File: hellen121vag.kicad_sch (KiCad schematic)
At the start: 35 parts, among them J21 Conn_01x05_Male, J22 USB_B_Mini, M1 Module-power_12and5V-0.3, M2 Module-knock-0.2, M3 Module-vr-discrete-0.5, M4 Module-vr-max9924-0.1, M5 Module-wbo-0.5, M6 Module:mega-mcu100/0.3, M7 Module-can-0.1, M8 Module-motor-driver-0.1, P1 368255-2, Q7 AO3400A, U10 BTS6143D

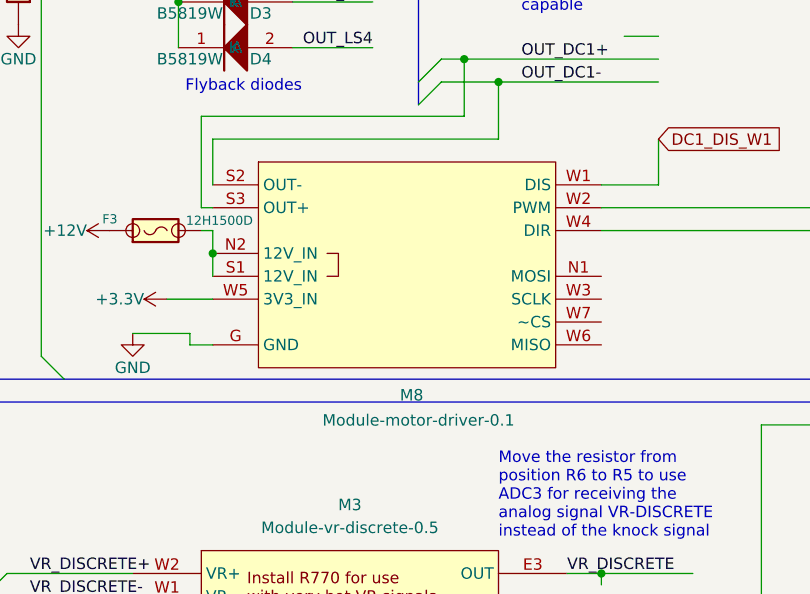
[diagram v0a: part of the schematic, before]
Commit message: sw
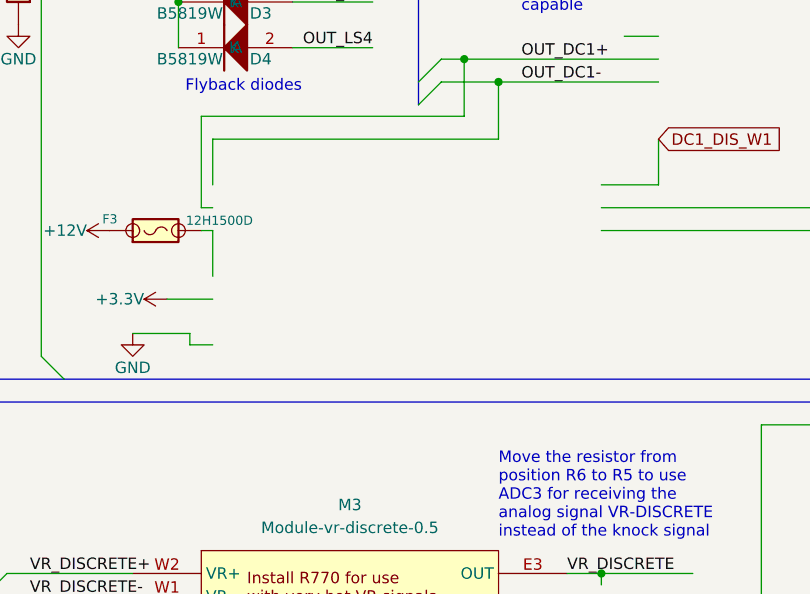
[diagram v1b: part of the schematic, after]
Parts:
- removed M8: Module-motor-driver-0.1, hellen-one-motor-driver-0.1:motor-driver, symbol motor-driver:Module-motor-driver-0.1
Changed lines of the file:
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@@
 	)
 	(junction
-		(at 209.55 201.93)
-		(diameter 0)
-		(color 0 0 0 0)
-	)
-	(junction
 		(at 205.74 163.83)
 		(diameter 0)
@@
 	(wire
 		(pts
-			(xy 209.55 201.93) (xy 209.55 204.47)
+			(xy 209.55 199.39) (xy 209.55 204.47)
 		)
 		(stroke
@@
 	(wire
 		(pts
-			(xy 209.55 199.39) (xy 209.55 201.93)
-		)
-		(stroke
-			(width 0)
-			(type default)
-		)
-	)
-	(wire
-		(pts
 			(xy 256.54 152.4) (xy 256.54 153.67)
 		)
@@
 					(unit 1)
 				)
-			)
-		)
-	)
-	(symbol
-		(lib_id "motor-driver:Module-motor-driver-0.1")
-		(at 214.63 191.77 0)
-		(unit 1)
-		(exclude_from_sim no)
-		(in_bom yes)
-		(on_board yes)
-		(dnp no)
-		(property "Reference" "M8"
-			(at 231.648 217.678 0)
-			(effects
-				(font
-					(size 1.27 1.27)
-				)
-			)
-		)
-		(property "Value" "Module-motor-driver-0.1"
-			(at 232.41 220.472 0)
-			(effects
-				(font
-					(size 1.27 1.27)
-				)
-			)
-		)
-		(property "Footprint" "hellen-one-motor-driver-0.1:motor-driver"
-			(at 240.03 190.5 0)
-			(effects
-				(font
-					(size 1.27 1.27)
-				)
-				(hide yes)
-			)
-		)
-		(property "Datasheet" ""
-			(at 214.63 191.77 0)
-			(effects
-				(font
-					(size 1.27 1.27)
-				)
-				(hide yes)
-			)
-		)
-		(property "Description" ""
-			(at 214.63 191.77 0)
-			(effects
-				(font
-					(size 1.27 1.27)
-				)
-				(hide yes)
-			)
-		)
-		(property "comentario" ""
-			(at 214.63 191.77 0)
-			(effects
-				(font
-					(size 1.27 1.27)
-				)
-				(hide yes)
-			)
-		)
-		(pin "W4"
-		)
-		(pin "N2"
-		)
-		(pin "N1"
-		)
-		(pin "G"
-		)
-		(pin "S2"
-		)
-		(pin "W2"
-		)
-		(pin "W7"
-		)
-		(pin "S3"
-		)
-		(pin "S1"
-		)
-		(pin "W6"
-		)
-		(pin "W1"
-		)
-		(pin "W5"
-		)
-		(pin "W3"
-		)
-		(instances
-			(project ""
-				(path "/45c1f041-3b7c-4036-abe9-e26621c05a73"
-					(reference "M8")
-					(unit 1)
-				)

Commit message: sw
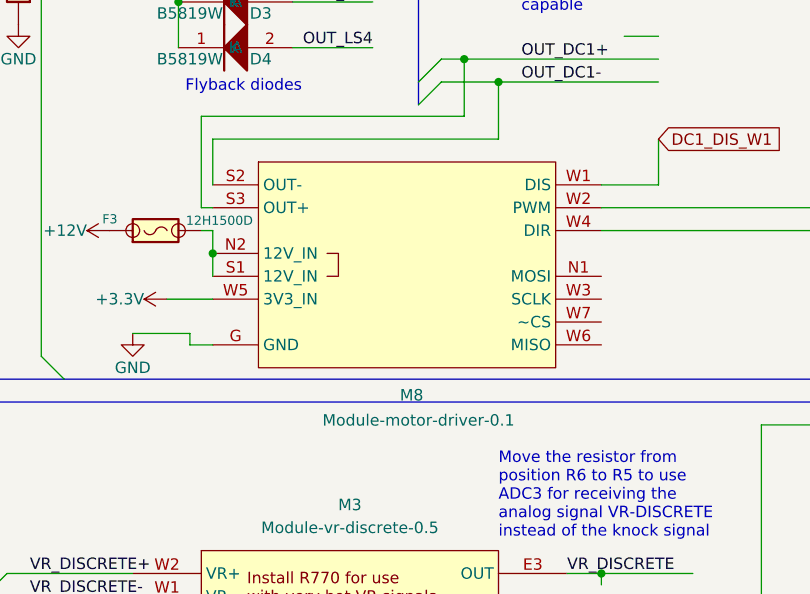
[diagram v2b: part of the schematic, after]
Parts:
- added M8: Module-motor-driver-0.1, hellen-one-motor-driver-0.1:motor-driver, symbol motor-driver:Module-motor-driver-0.1
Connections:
- net +3.3V: now also M8.W5 (3V3_IN)
- net DC1_DIR: now also M8.W4 (DIR)
- net DC1_DIS_W1: now also M8.W1 (DIS)
- net DC1_PWM: now also M8.W2 (PWM)
- net GND: now also M8.G (GND)
- net PIN1: now also M8.S3 (OUT+)
- net PIN2: now also M8.S2 (OUT-)
- net at F3.2: now also M8.N2 (12V_IN), M8.S1 (12V_IN)
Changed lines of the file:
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@@
 	)
 	(junction
+		(at 209.55 201.93)
+		(diameter 0)
+		(color 0 0 0 0)
+	)
+	(junction
 		(at 205.74 163.83)
 		(diameter 0)
@@
 	(wire
 		(pts
-			(xy 209.55 199.39) (xy 209.55 204.47)
+			(xy 209.55 201.93) (xy 209.55 204.47)
 		)
 		(stroke
@@
 	(wire
 		(pts
+			(xy 209.55 199.39) (xy 209.55 201.93)
+		)
+		(stroke
+			(width 0)
+			(type default)
+		)
+	)
+	(wire
+		(pts
 			(xy 256.54 152.4) (xy 256.54 153.67)
 		)
@@
 					(unit 1)
 				)
+			)
+		)
+	)
+	(symbol
+		(lib_id "motor-driver:Module-motor-driver-0.1")
+		(at 214.63 191.77 0)
+		(unit 1)
+		(exclude_from_sim no)
+		(in_bom yes)
+		(on_board yes)
+		(dnp no)
+		(property "Reference" "M8"
+			(at 231.648 217.678 0)
+			(effects
+				(font
+					(size 1.27 1.27)
+				)
+			)
+		)
+		(property "Value" "Module-motor-driver-0.1"
+			(at 232.41 220.472 0)
+			(effects
+				(font
+					(size 1.27 1.27)
+				)
+			)
+		)
+		(property "Footprint" "hellen-one-motor-driver-0.1:motor-driver"
+			(at 240.03 190.5 0)
+			(effects
+				(font
+					(size 1.27 1.27)
+				)
+				(hide yes)
+			)
+		)
+		(property "Datasheet" ""
+			(at 214.63 191.77 0)
+			(effects
+				(font
+					(size 1.27 1.27)
+				)
+				(hide yes)
+			)
+		)
+		(property "Description" ""
+			(at 214.63 191.77 0)
+			(effects
+				(font
+					(size 1.27 1.27)
+				)
+				(hide yes)
+			)
+		)
+		(property "comentario" ""
+			(at 214.63 191.77 0)
+			(effects
+				(font
+					(size 1.27 1.27)
+				)
+				(hide yes)
+			)
+		)
+		(pin "W4"
+		)
+		(pin "N2"
+		)
+		(pin "N1"
+		)
+		(pin "G"
+		)
+		(pin "S2"
+		)
+		(pin "W2"
+		)
+		(pin "W7"
+		)
+		(pin "S3"
+		)
+		(pin "S1"
+		)
+		(pin "W6"
+		)
+		(pin "W1"
+		)
+		(pin "W5"
+		)
+		(pin "W3"
+		)
+		(instances
+			(project ""
+				(path "/45c1f041-3b7c-4036-abe9-e26621c05a73"
+					(reference "M8")
+					(unit 1)
+				)
